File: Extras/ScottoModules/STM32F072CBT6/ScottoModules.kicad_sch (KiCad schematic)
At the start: 30 parts, among them J1 USB_C, SW1 SW_Push, U1 STM32F072CBT6, U3 XC6206, U4 USBLC6-2SC6

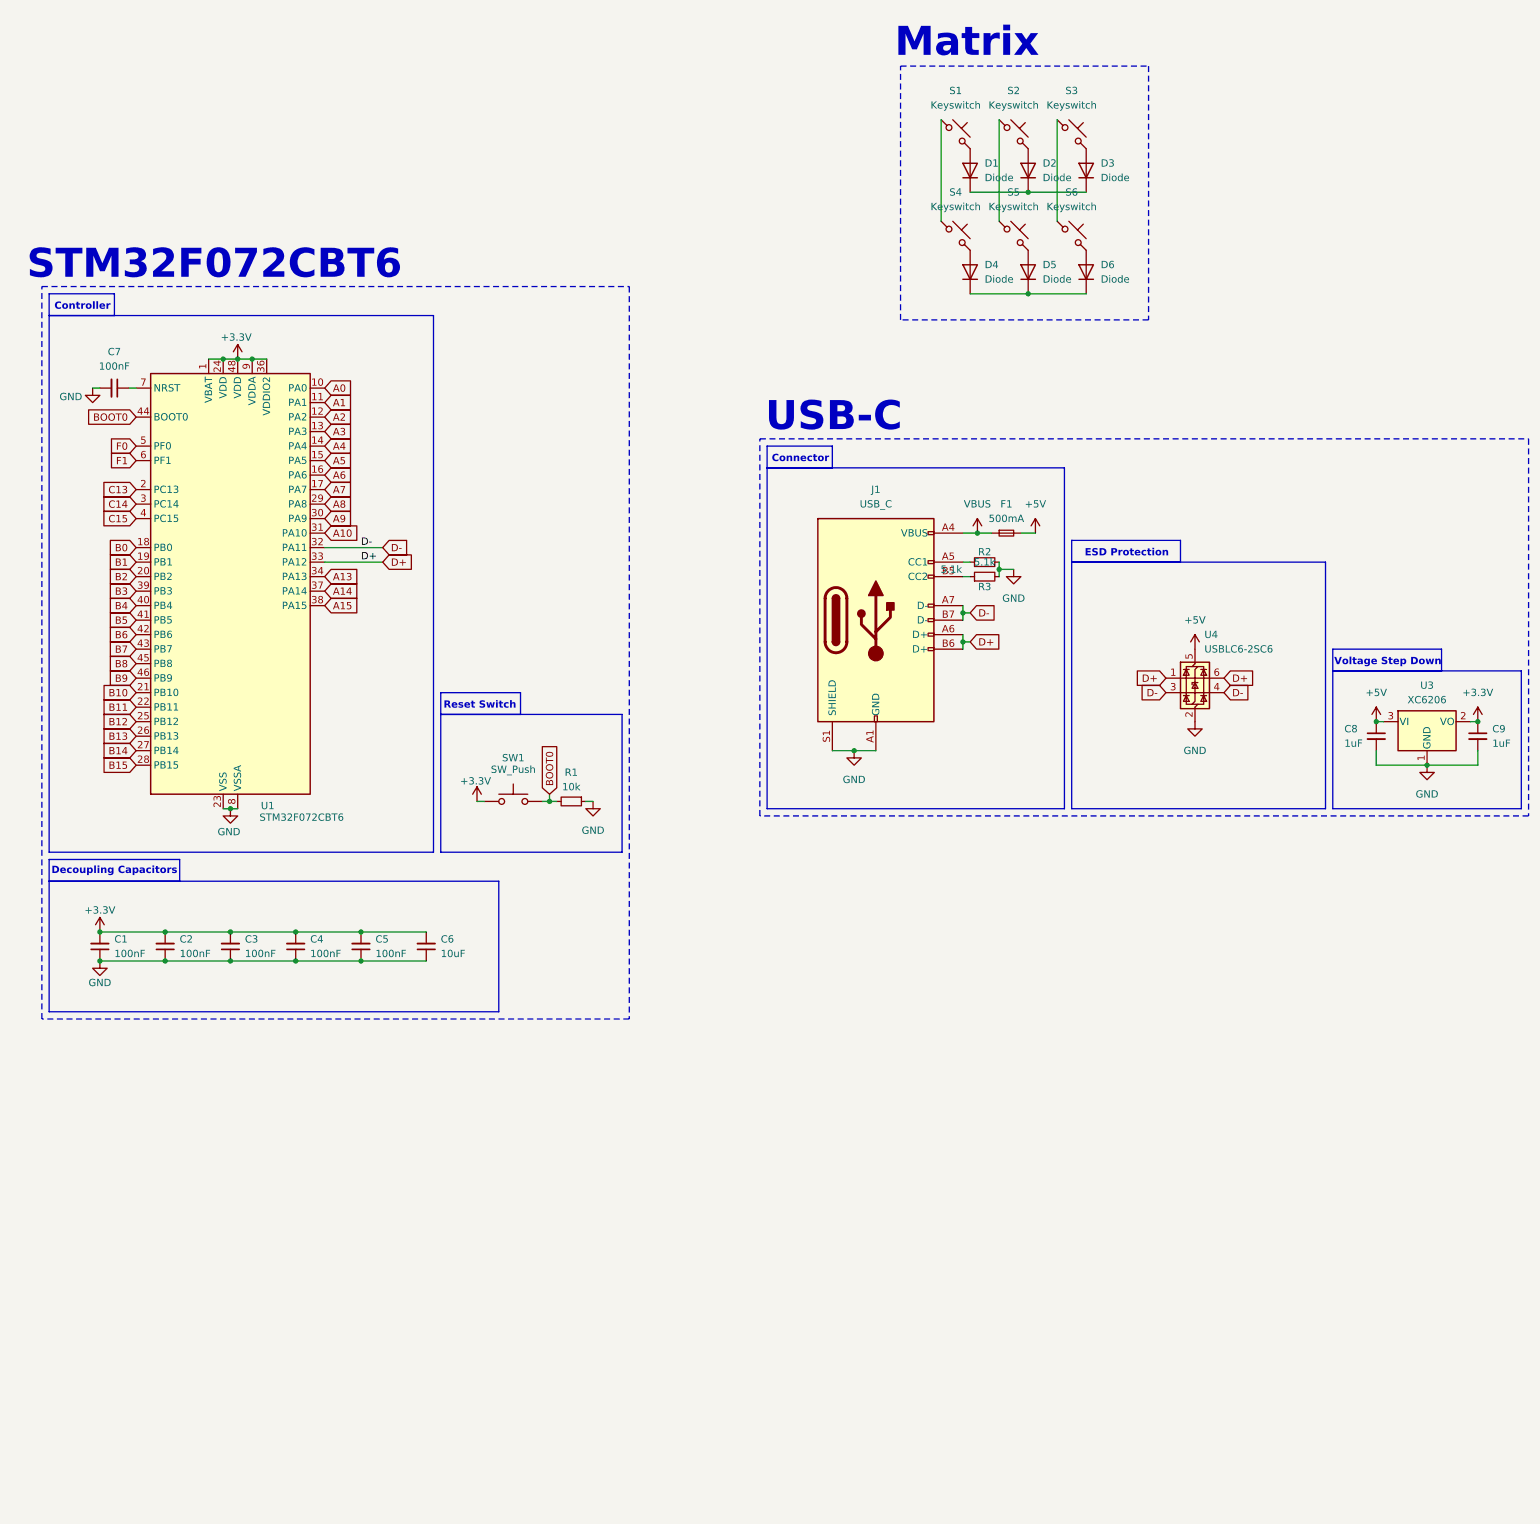
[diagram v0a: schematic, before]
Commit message: Add Template
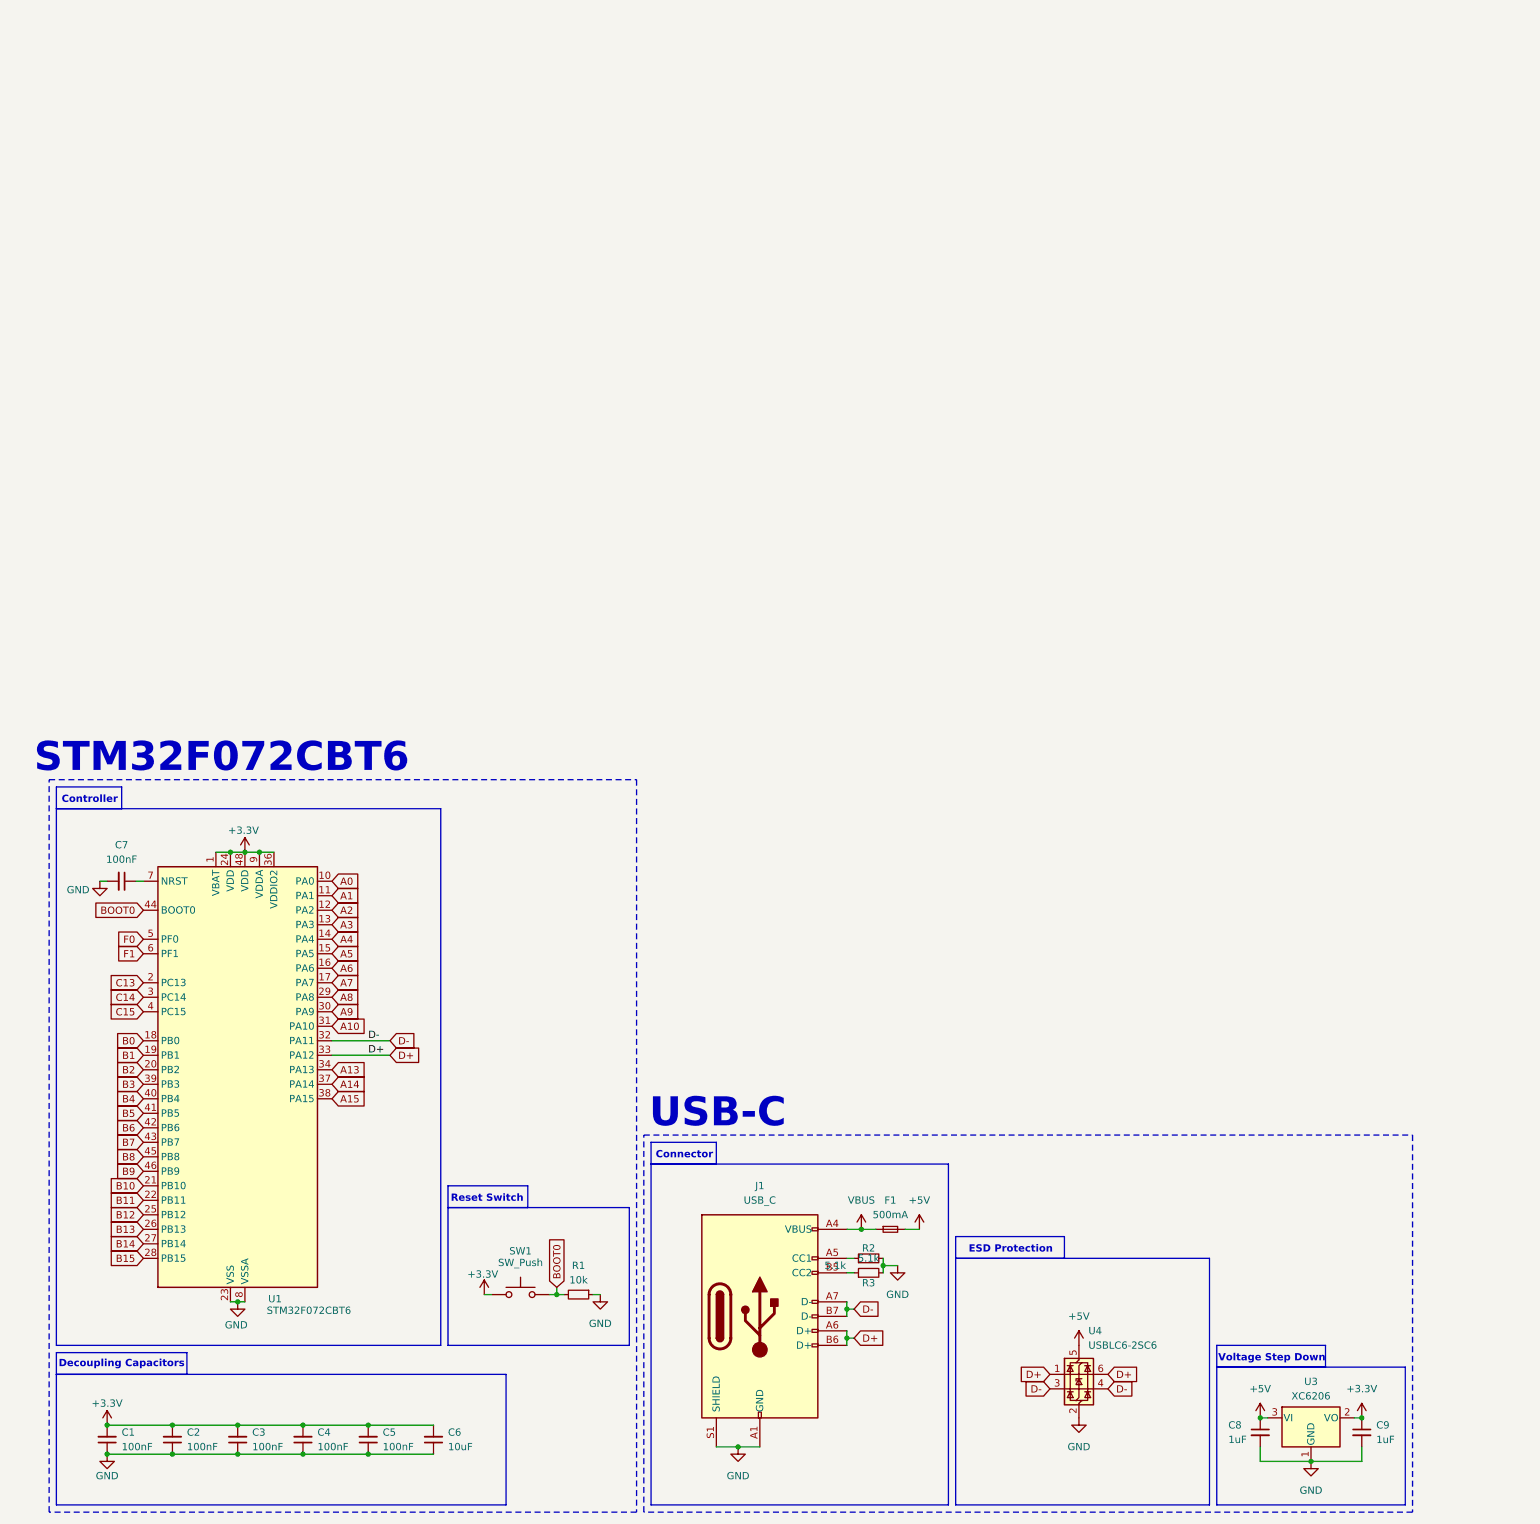
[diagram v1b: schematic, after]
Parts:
- removed D1, D2, D3, D4, D5, D6: Diode, ScottoKeebs_Components:Diode_SOD-123, symbol ScottoKeebs:Placeholder_Diode
- removed S1, S2, S3, S4, S5, S6: Keyswitch, ScottoKeebs_Scotto:MX_1.00u, symbol ScottoKeebs:Placeholder_Keyswitch
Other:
- note removed: "Matrix"
- moved on the sheet: C1, C2, C3, C4, C5, C6, C7, C8, C9, F1, J1, R1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
